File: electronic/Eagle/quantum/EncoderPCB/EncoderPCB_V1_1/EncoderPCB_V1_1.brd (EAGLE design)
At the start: 30 x 60 mm, 27 parts, among them IC1 STM32F031K6T6, J1 90814-0204

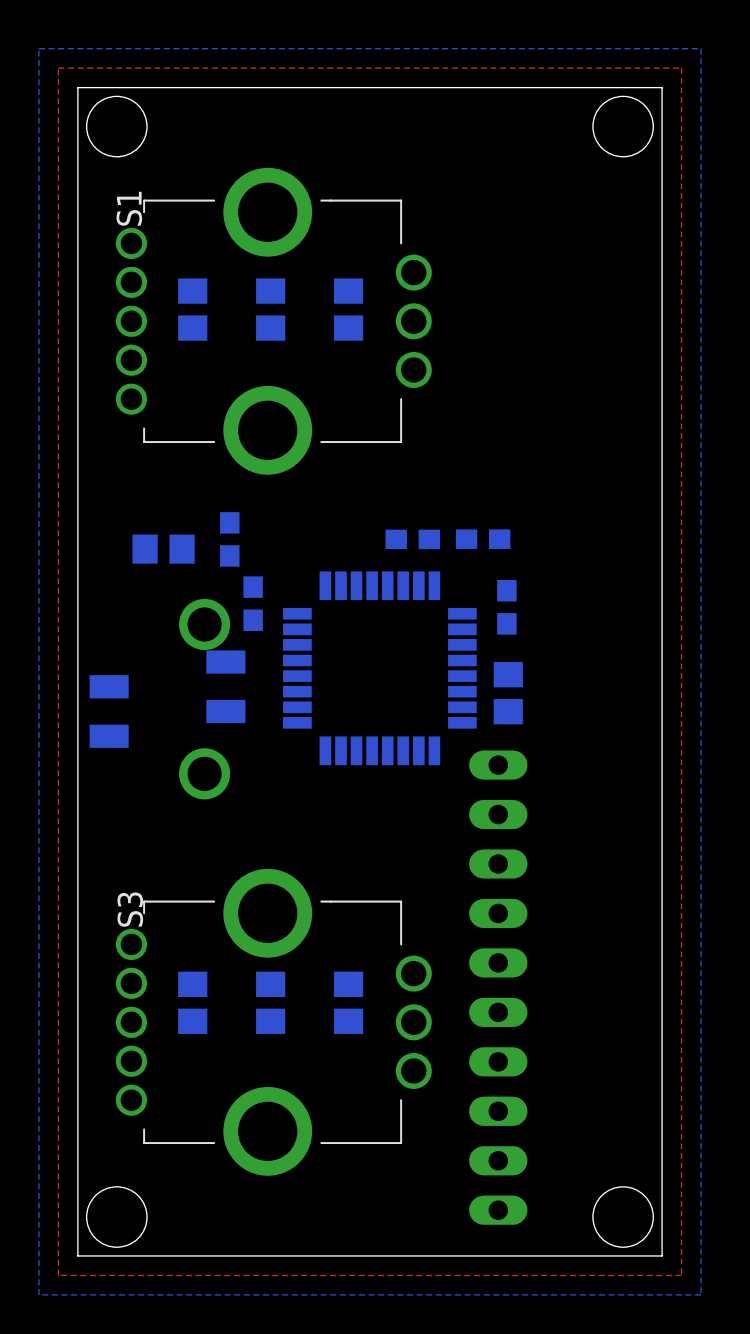
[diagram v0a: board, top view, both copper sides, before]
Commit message: Encoder_v1_1 changes
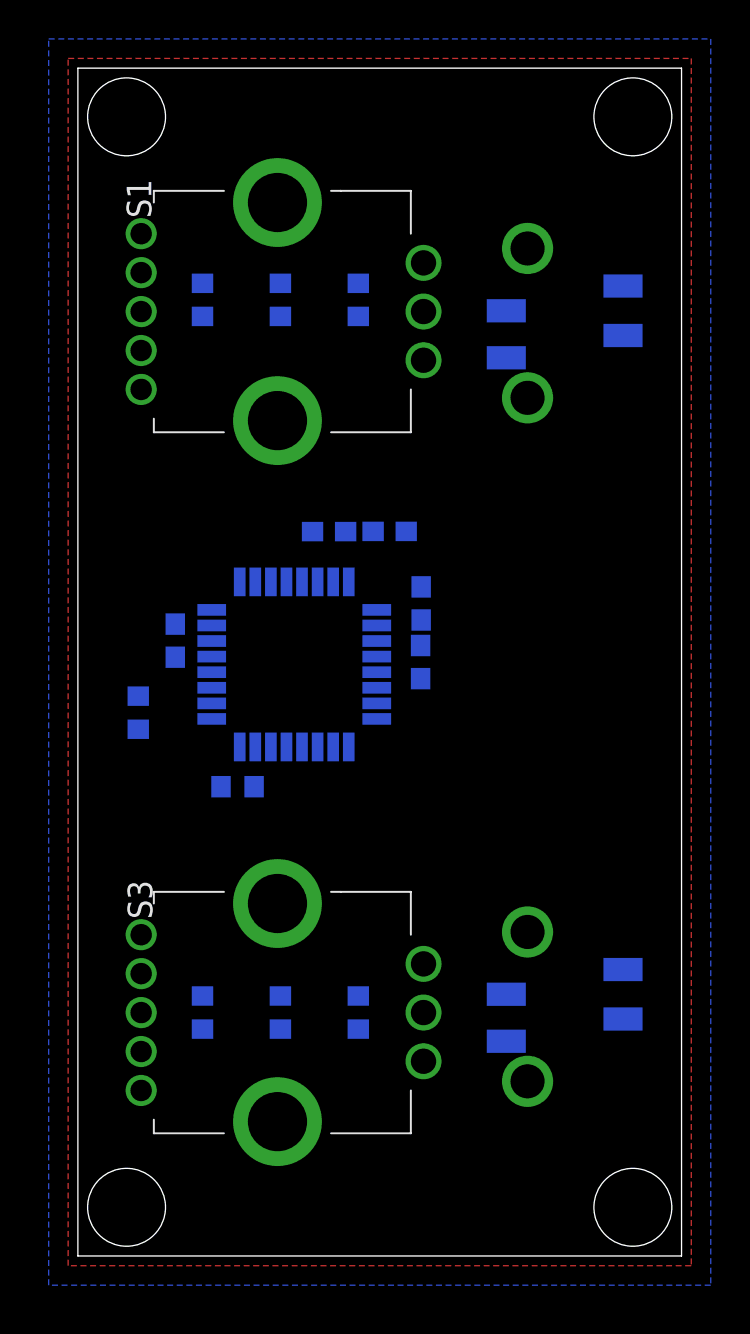
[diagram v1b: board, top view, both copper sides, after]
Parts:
- removed 3V1, GND, GND2, I2C1_SCL, I2C1_SDA, NRST, SWCLK, SWDIO, USART1_RX1, USART1_TX: TPTHT, C_Sager_Bibliothek:THT_PIN
- removed J1: 90814-0204, electro_mechanical:MOLEX_90814-0204
- added I2C-CONN, PRG-CONN: 90814-0204, electro_mechanical:MOLEX_90814-0204
- R1, R11: device C_Sager_Bibliothek:R0805 -> passive components:R0603
- R10, R2, R3, R4, R8, R9: value (none) -> 51 R; device C_Sager_Bibliothek:R0805 -> passive components:R0603
- moved R11 14.7 mm to (8.20, 24.1), turned to 180 degrees
- moved C1 11.7 mm to (17.6, 30.5)
- moved R1 8.50 mm to (3.10, 27.9), turned to 270 degrees
- moved C4 4.82 mm to (16.0, 37.2)
- moved C2 4.43 mm to (5.00, 31.6)
- moved C3 4.40 mm to (17.6, 33.5)
- moved IC1 4.40 mm to (11.1, 30.4)
- moved C5 4.32 mm to (12.9, 37.2)
- moved R10 0.71 mm to (6.40, 12.5)
- moved R2 0.71 mm to (14.4, 49.1)
- moved R3 0.71 mm to (10.4, 49.1)
- moved R4 0.71 mm to (6.40, 49.1)
- moved R8 0.71 mm to (14.4, 12.5)
- moved R9 0.71 mm to (10.4, 12.5)
- moved S1 0.71 mm to (10.5, 48.5)
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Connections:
- net +3V3: now also I2C-CONN.3; no longer 3V1.P$1
- net GND: now also I2C-CONN.4, PRG-CONN.4; no longer GND.P$1, GND2.P$1
- net I2C1_SCL: now also I2C-CONN.2; no longer I2C1_SCL.P$1
- net I2C1_SDA: now also I2C-CONN.1; no longer I2C1_SDA.P$1
- net NRST: now also PRG-CONN.2; no longer NRST.P$1
- net SWCLK: now also PRG-CONN.1; no longer SWCLK.P$1
- net SWDIO: now also PRG-CONN.3; no longer SWDIO.P$1
- net USART1_RX1: no longer USART1_RX1.P$1
- net USART1_TX: no longer USART1_TX.P$1
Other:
- board size 30 x 60 mm -> 31 x 61 mm
- board text removed: "+3V3"
- board text removed: "GND"
- board text removed: "NRST"
- board text removed: "RX"
- board text removed: "SCL"
- board text removed: "SDA"
- board text removed: "SWCLK"
- board text removed: "SWDIO"
- board text removed: "TX"
